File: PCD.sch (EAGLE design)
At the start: 23 parts, among them IC2 TCAN332DR, IC4 MCP2515, J1 M40-SOCKET-BELOW, J2 DC IN, J4 DC IN, J5 CAN Termination

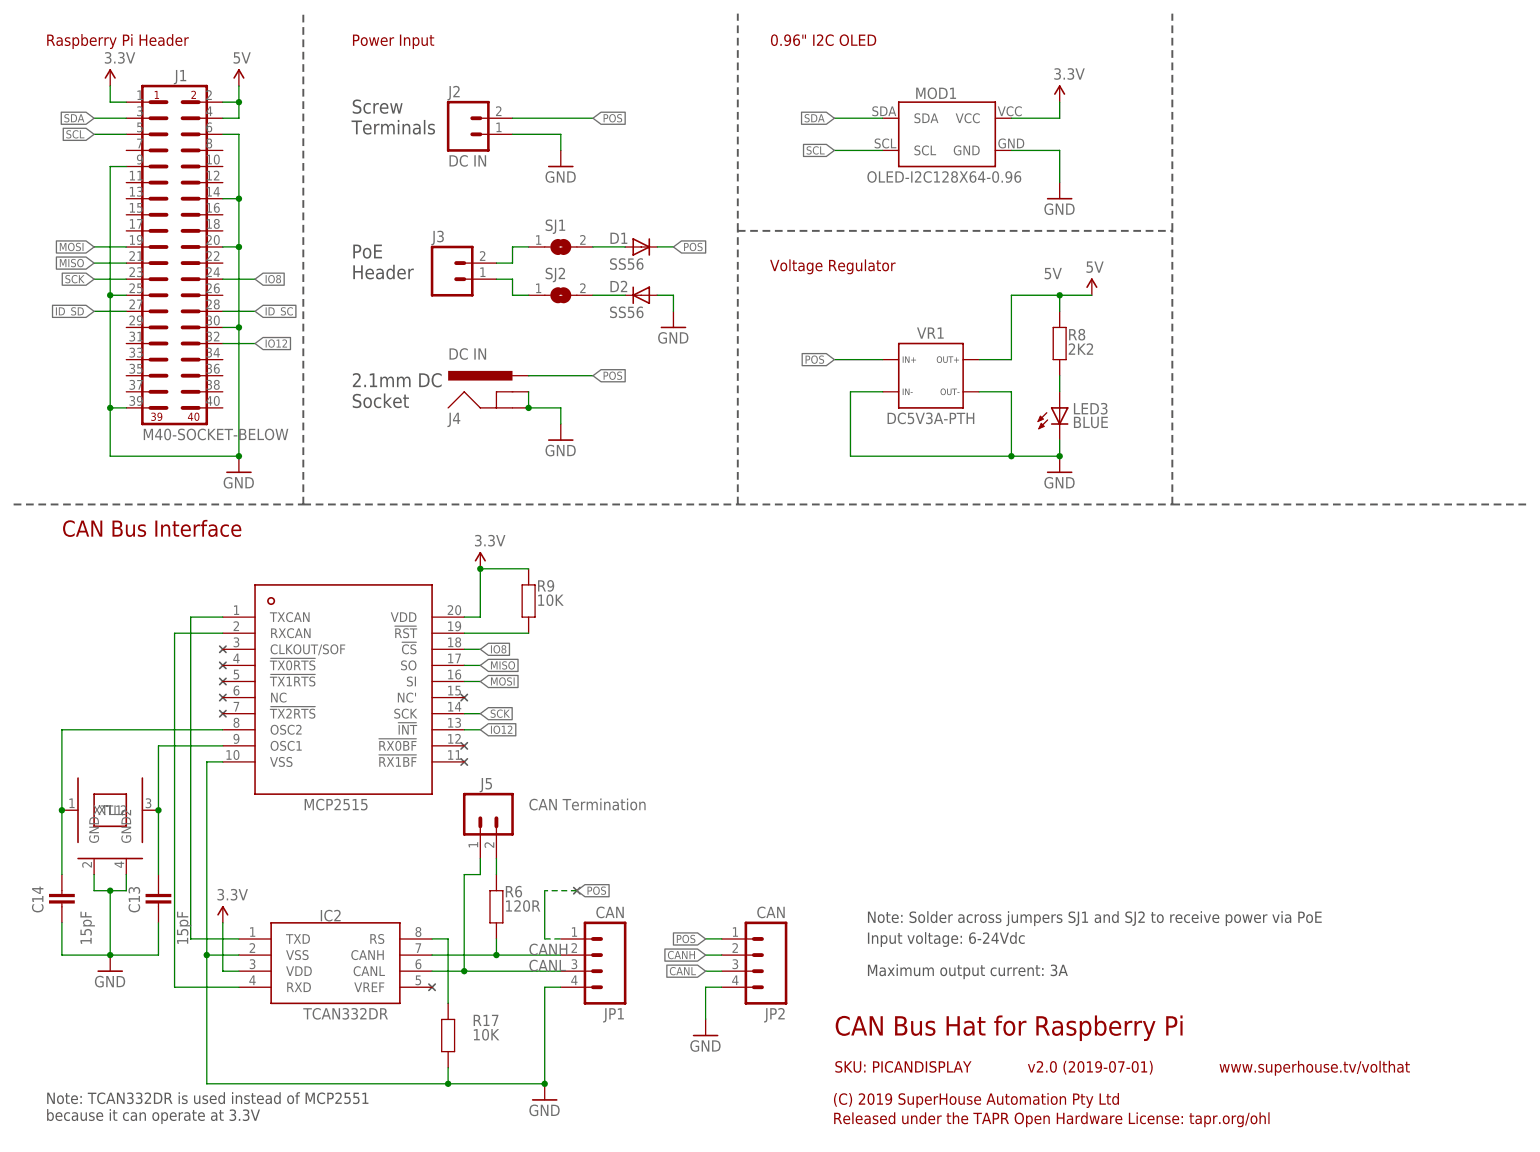
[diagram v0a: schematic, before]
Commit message: Major work for v1.0 release
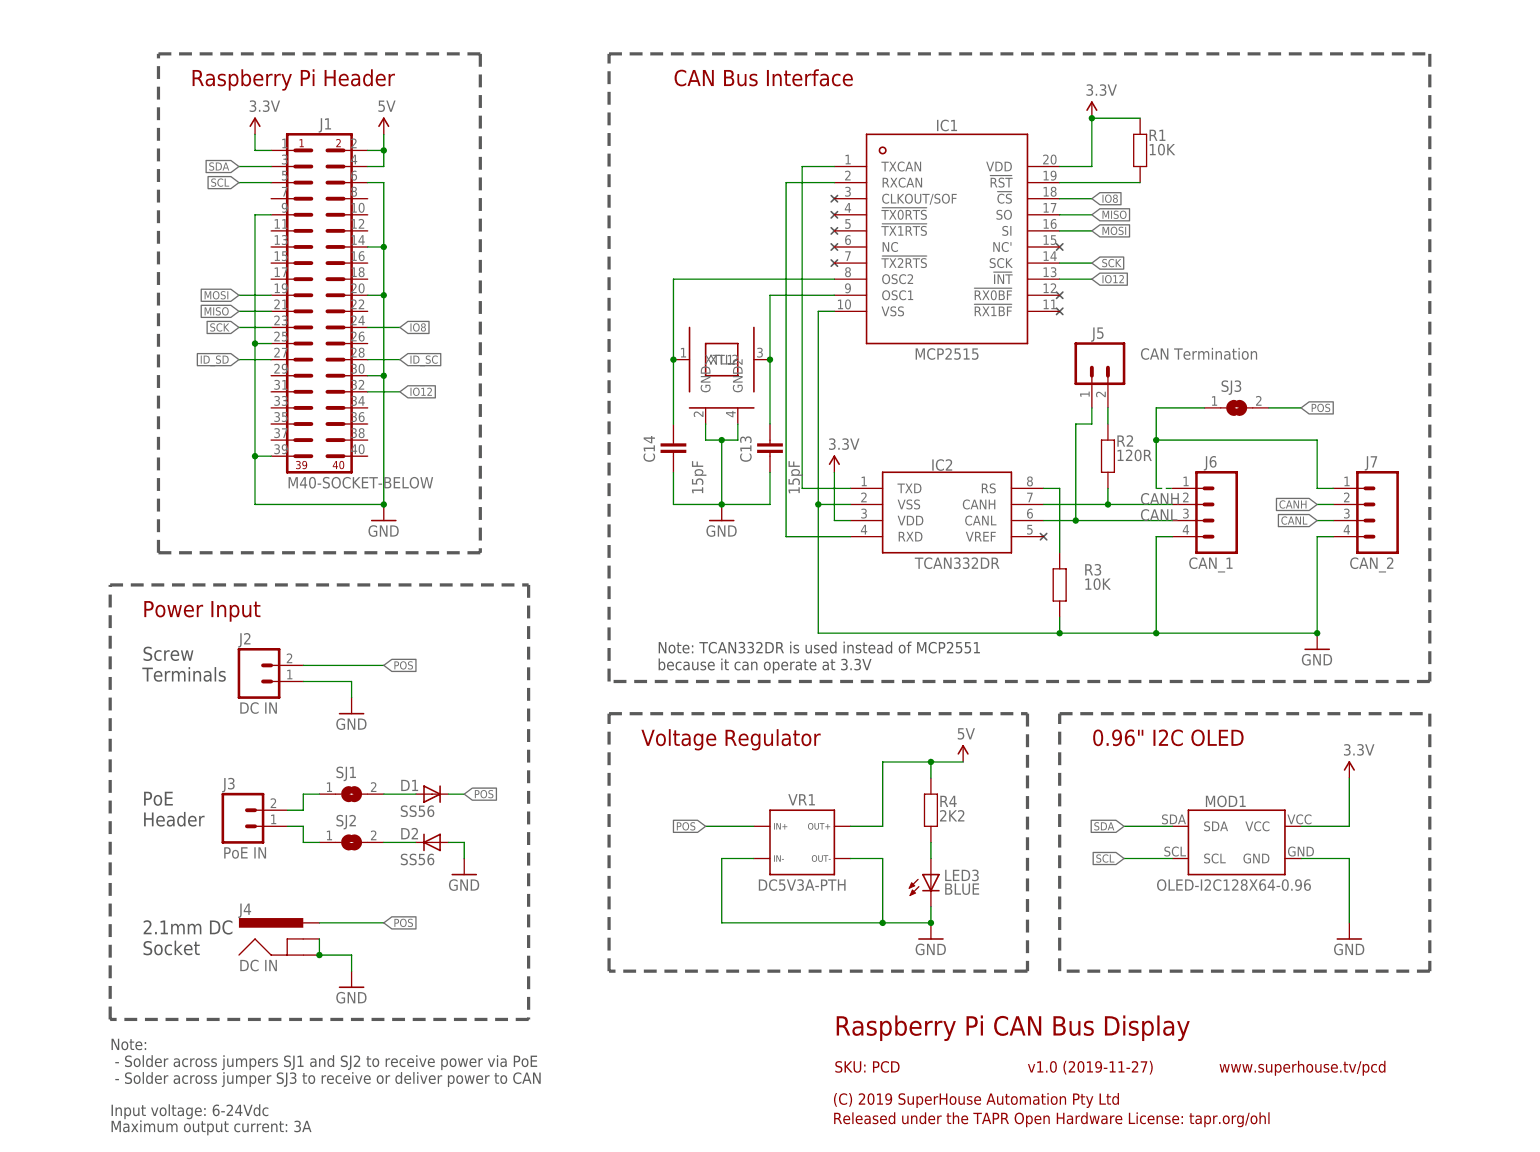
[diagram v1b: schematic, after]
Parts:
- removed IC4: MCP2515, SuperHouse-ICs:MCP2515
- removed JP1, JP2: CAN, SuperHouse-Connectors:M04-PIN
- removed R17, R9: 10K, SuperHouse-DiscreteSemi:RESISTOR0603
- removed R6: 120R, SuperHouse-DiscreteSemi:RESISTOR0603
- removed R8: 2K2, SuperHouse-DiscreteSemi:RESISTOR0603
- added IC1: MCP2515, SuperHouse-ICs:MCP2515
- added J6: CAN_1, SuperHouse-Connectors:M04-PIN
- added J7: CAN_2, SuperHouse-Connectors:M04-PIN
- added R1, R3: 10K, SuperHouse-DiscreteSemi:RESISTOR0603
- added R2: 120R, SuperHouse-DiscreteSemi:RESISTOR0603
- added R4: 2K2, SuperHouse-DiscreteSemi:RESISTOR0603
- added SJ3: (no value), freetronics-jon:SJN
- J3: value (none) -> PoE IN
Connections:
- new net CAN_PWR: J6.1, J7.1, SJ3.1
- net 3.3V: now also IC1.VDD, R1.2; no longer IC4.VDD, R9.2
- net 5V: now also R4.1; no longer R8.1
- net CANH: now also J6.2, J7.2, R2.1; no longer JP1.2, JP2.2, R6.1
- net CANL: now also J6.3, J7.3; no longer JP1.3, JP2.3
- net GND: now also IC1.VSS, J6.4, J7.4, R3.1; no longer IC4.VSS, JP1.4, JP2.4, R17.1
- net IO12: now also IC1.!INT; no longer IC4.!INT
- net IO8: now also IC1.!CS; no longer IC4.!CS
- net MISO: now also IC1.SO; no longer IC4.SO
- net MOSI: now also IC1.SI; no longer IC4.SI
- net N$203: now also R4.2; no longer R8.2
- net N$26: now also R3.2; no longer R17.2
- net N$28: now also IC1.TXCAN; no longer IC4.TXCAN
- net N$29: now also IC1.RXCAN; no longer IC4.RXCAN
- net N$3: now also R2.2; no longer R6.2
- net N$30: now also IC1.OSC1; no longer IC4.OSC1
- net N$48: now also IC1.OSC2; no longer IC4.OSC2
- net N$49: now also IC1.!RST, R1.1; no longer IC4.!RST, R9.1
- net POS: now also SJ3.2; no longer JP1.1, JP2.1
- net SCK: now also IC1.SCK; no longer IC4.SCK
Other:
- note added: "Note: - Solder across jumpers SJ1 and SJ2 to receive power via PoE - Solder across jumper SJ3 to receive or deliver power to CAN"
- note added: "Raspberry Pi CAN Bus Display"
- note added: "SKU: PCD"
- note added: "v1.0 (2019-11-27)"
- note added: "www.superhouse.tv/pcd"
- note removed: "CAN Bus Hat for Raspberry Pi"
- note removed: "Note: Solder across jumpers SJ1 and SJ2 to receive power via PoE"
- note removed: "SKU: PICANDISPLAY"
- note removed: "v2.0 (2019-07-01)"
- note removed: "www.superhouse.tv/volthat"
- moved on the sheet: C13, C14, D1, D2, IC2, J1, J2, J3, J4, J5, LED3, MOD1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
